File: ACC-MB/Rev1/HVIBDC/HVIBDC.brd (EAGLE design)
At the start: 100.2 x 48.2 mm, 34 parts, among them IC1 555

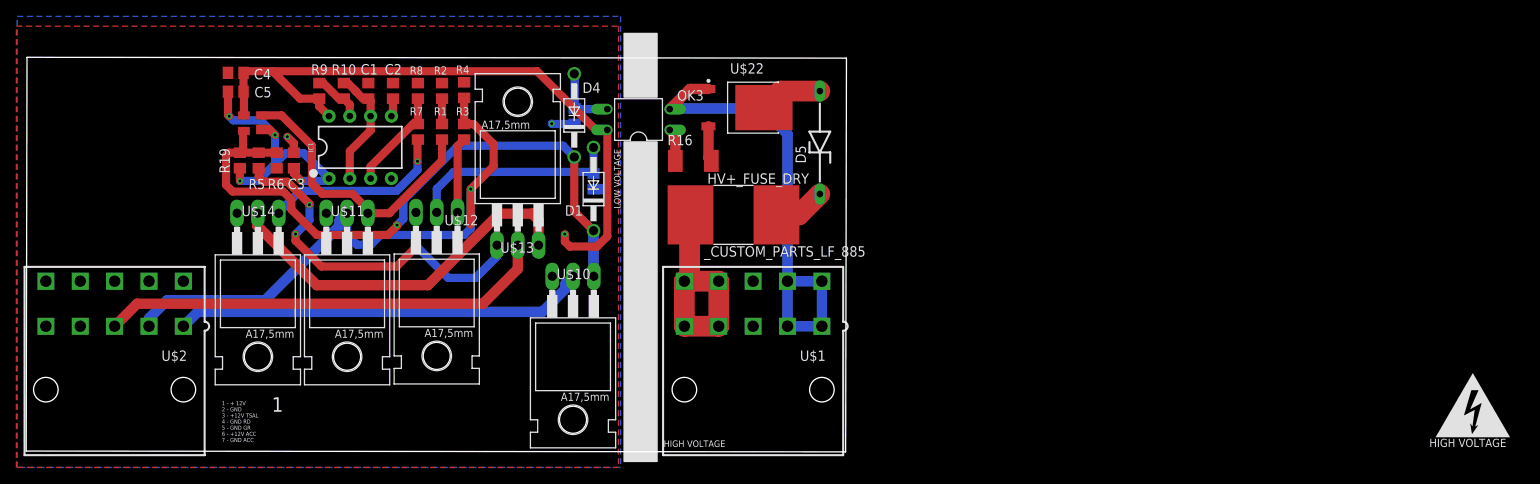
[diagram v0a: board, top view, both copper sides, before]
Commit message: update
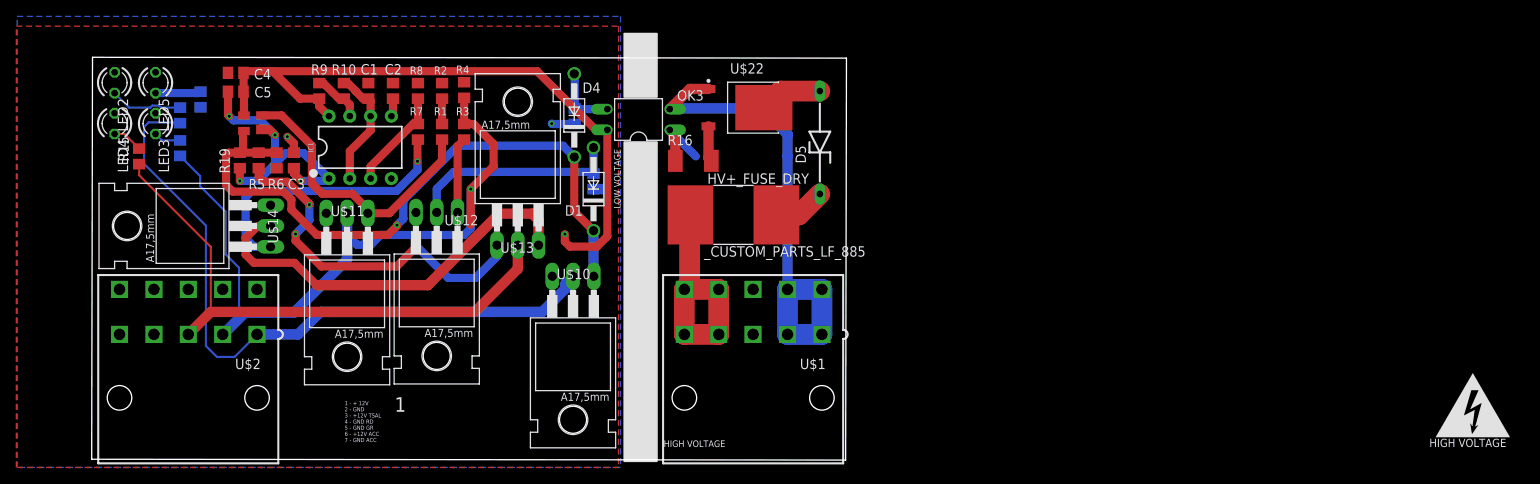
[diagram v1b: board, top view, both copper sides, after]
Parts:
- added LED2, LED3, LED4, LED5: (no value), ACC-MB-R0:LED3MM
- added R13, R14, R15, R18: (no value), ACC-MB-R0:R0805
- moved U$2 9.06 mm to (-3.00, 17.0)
- moved U$14 6.79 mm to (0.70, 27.5), turned to 90 degrees
- moved U$1 1.00 mm to (66.0, 17.0)
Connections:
- new net N$17: LED2.K, R13.2
- new net N$19: LED3.K, R14.2
- new net N$25: LED4.K, R15.2
- new net N$27: LED5.K, R18.2
- net +12V: now also LED2.A, LED3.A, LED4.A, LED5.A
- net ACC_LGHT: now also R13.1
- net GND: now also R18.1
- net TSAL_GRN_GND: now also R14.1
- net TSAL_RED_GND: now also R15.1
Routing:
- net ACC_LGHT: track 50.5 -> 84.4 mm
- net TSAL_GRN_GND: track 73.5 -> 89.8 mm
- net TSAL_RED_GND: track 55.0 -> 68.1 mm
- net N$7: track 22.9 -> 34.6 mm
- net N$17: track 0.00 -> 8.95 mm
- net N$27: track 0.00 -> 5.57 mm
- net N$22: track 4.07 -> 8.62 mm
- net N$13: track 45.9 -> 50.0 mm
- net N$25: track 0.00 -> 3.74 mm
- net N$19: track 0.00 -> 3.32 mm
- net V-: track 58.9 -> 59.9 mm
- net V+: track 27.8 -> 28.8 mm
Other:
- board size 100.2 x 48.2 mm -> 92.2 x 49.2 mm
